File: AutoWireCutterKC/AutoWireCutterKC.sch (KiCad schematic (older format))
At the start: 17 parts, among them J1 LCD I/O, J2 ISP, J3 LCD Serial, J5 LCD Power, J6 Servo, J8 Barrel_Jack, J9 Stepper, U1 ATMEGA328P-AU, U2 MCP1700_SOT23, U3 LT1129-5.0_SOT223

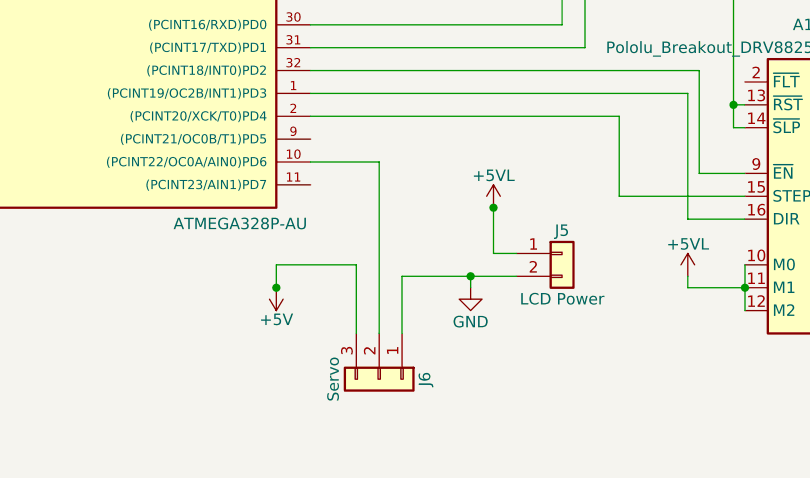
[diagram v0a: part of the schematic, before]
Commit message: PCB Populated
Traces needed
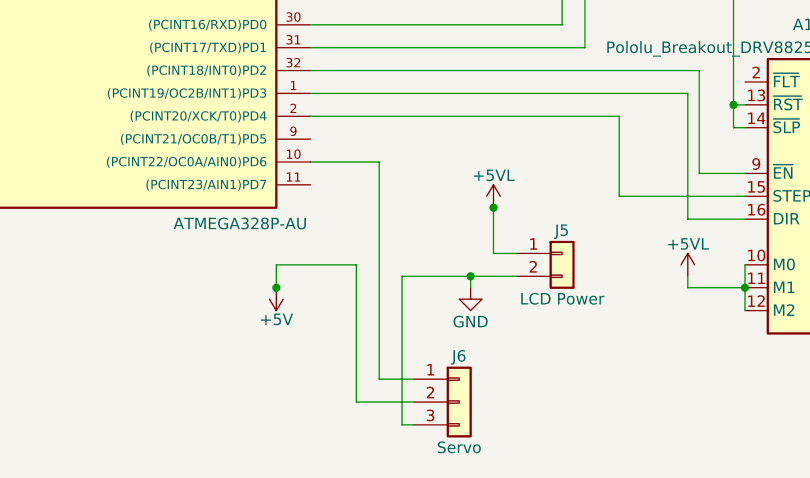
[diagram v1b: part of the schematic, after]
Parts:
- C1, C3, C4, C5: footprint (none) -> Capacitors_SMD:C_0805_HandSoldering
- C2: footprint (none) -> Capacitors_SMD:CP_Elec_6.3x7.7
- C6: footprint (none) -> Capacitors_Tantalum_SMD:CP_Tantalum_Case-B_EIA-3528-21_Hand
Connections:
- net +5V: now also J6.2 (Pin_2); no longer J6.3 (Pin_3)
- net GND: now also J6.3 (Pin_3); no longer J6.1 (Pin_1)
- net at U1.10 ((PCINT22/OC0A/AIN0)PD6): now also J6.1 (Pin_1); no longer J6.2 (Pin_2)
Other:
- moved on the sheet: J6
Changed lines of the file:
@@
 LIBS:valves
 LIBS:Driver_Motor
+LIBS:pololu-drv8825
 LIBS:AutoWireCutterKC-cache
 EELAYER 25 0
@@
 F 0 "C1" H 1425 4650 50  0000 L CNN
 F 1 "100n" H 1425 4450 50  0000 L CNN
-F 2 "" H 1438 4400 50  0001 C CNN
+F 2 "Capacitors_SMD:C_0805_HandSoldering" H 1438 4400 50  0001 C CNN
 F 3 "" H 1400 4550 50  0001 C CNN
 	1    1400 4550
@@
 F 0 "C2" H 6175 4300 50  0000 L CNN
 F 1 "100u" H 6175 4100 50  0000 L CNN
-F 2 "" H 6188 4050 50  0001 C CNN
+F 2 "Capacitors_SMD:CP_Elec_6.3x7.7" H 6188 4050 50  0001 C CNN
 F 3 "" H 6150 4200 50  0001 C CNN
 	1    6150 4200
@@
 L Conn_01x03 J6
 U 1 1 5B1AA4B7
-P 3750 5900
-F 0 "J6" H 3750 6100 50  0000 C CNN
-F 1 "Servo" H 3750 5700 50  0000 C CNN
-F 2 "Pin_Headers:Pin_Header_Angled_1x03_Pitch2.54mm" H 3750 5900 50  0001 C CNN
-F 3 "" H 3750 5900 50  0001 C CNN
-	1    3750 5900
-	0    1    1    0
+P 4100 6000
+F 0 "J6" H 4100 6200 50  0000 C CNN
+F 1 "Servo" H 4100 5800 50  0000 C CNN
+F 2 "Pin_Headers:Pin_Header_Angled_1x03_Pitch2.54mm" H 4100 6000 50  0001 C CNN
+F 3 "" H 4100 6000 50  0001 C CNN
+	1    4100 6000
+	1    0    0    -1
 $EndComp
 $Comp
@@
 F 0 "C3" H 8475 4750 50  0000 L CNN
 F 1 "1u" H 8475 4550 50  0000 L CNN
-F 2 "" H 8488 4500 50  0001 C CNN
+F 2 "Capacitors_SMD:C_0805_HandSoldering" H 8488 4500 50  0001 C CNN
 F 3 "" H 8450 4650 50  0001 C CNN
 	1    8450 4650
@@
 F 0 "C5" H 8525 3950 50  0000 L CNN
 F 1 "1u" H 8525 3750 50  0000 L CNN
-F 2 "" H 8538 3700 50  0001 C CNN
+F 2 "Capacitors_SMD:C_0805_HandSoldering" H 8538 3700 50  0001 C CNN
 F 3 "" H 8500 3850 50  0001 C CNN
 	1    8500 3850
@@
 F 0 "C4" H 9325 4750 50  0000 L CNN
 F 1 "1u" H 9325 4550 50  0000 L CNN
-F 2 "" H 9338 4500 50  0001 C CNN
+F 2 "Capacitors_SMD:C_0805_HandSoldering" H 9338 4500 50  0001 C CNN
 F 3 "" H 9300 4650 50  0001 C CNN
 	1    9300 4650
@@
 F 0 "C6" H 9425 3950 50  0000 L CNN
 F 1 "3.3u" H 9425 3750 50  0000 L CNN
-F 2 "" H 9400 3850 50  0001 C CNN
+F 2 "Capacitors_Tantalum_SMD:CP_Tantalum_Case-B_EIA-3528-21_Hand" H 9400 3850 50  0001 C CNN
 F 3 "" H 9400 3850 50  0001 C CNN
 	1    9400 3850
@@
 	3450 4950 3750 4950
 Wire Wire Line
-	3750 4950 3750 5700
-Wire Wire Line
-	3850 5700 3850 5450
+	3750 4950 3750 5900
+Wire Wire Line
+	3850 5450 3850 6100
 Connection ~ 4150 5450
 Wire Wire Line
-	3650 5700 3650 5400
+	3650 5400 3650 6000
 Wire Wire Line
 	3650 5400 3300 5400
@@
 Wire Wire Line
 	5300 4150 5300 4800
+Wire Wire Line
+	3750 5900 3900 5900
+Wire Wire Line
+	3650 6000 3900 6000
+Wire Wire Line
+	3850 6100 3900 6100
 $EndSCHEMATC
